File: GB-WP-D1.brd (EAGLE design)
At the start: 39.7 x 44.1 mm, 9 parts

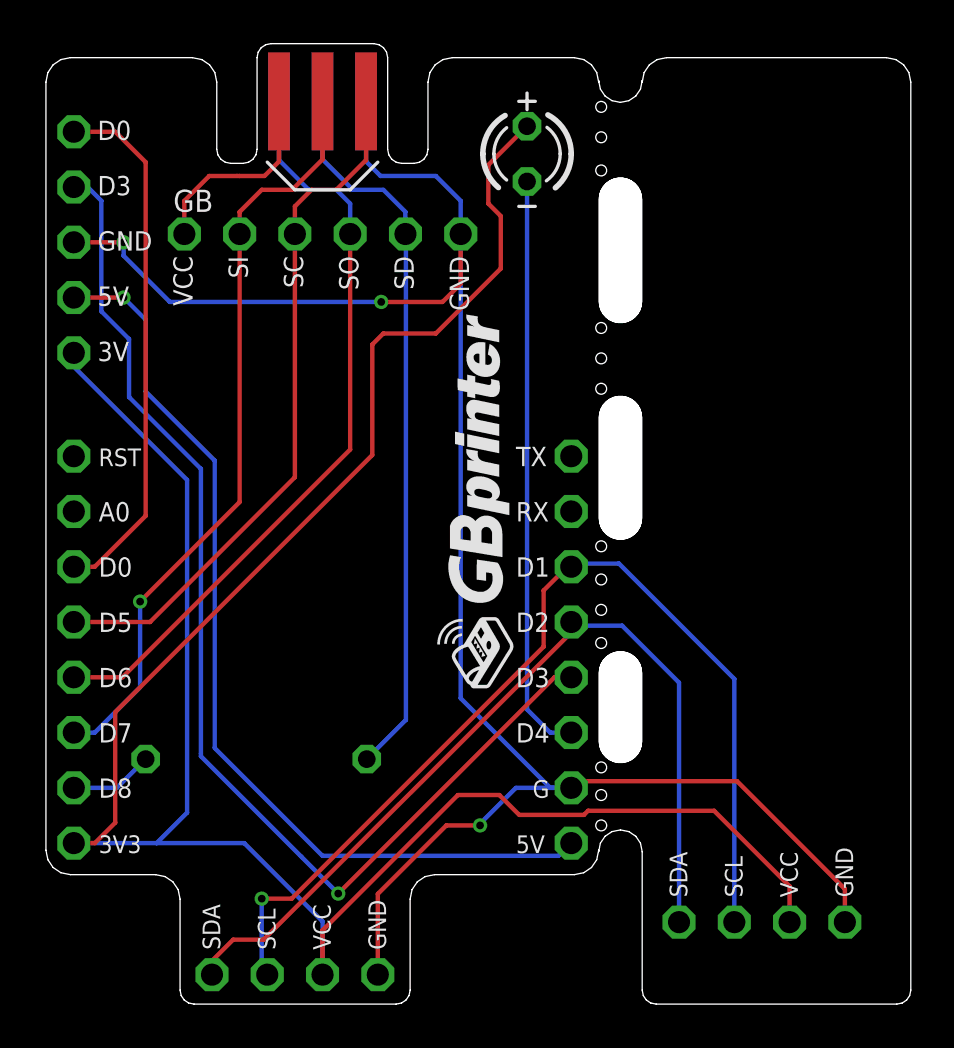
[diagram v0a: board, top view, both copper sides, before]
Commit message: Add files via upload
WEMOS D1 mini size
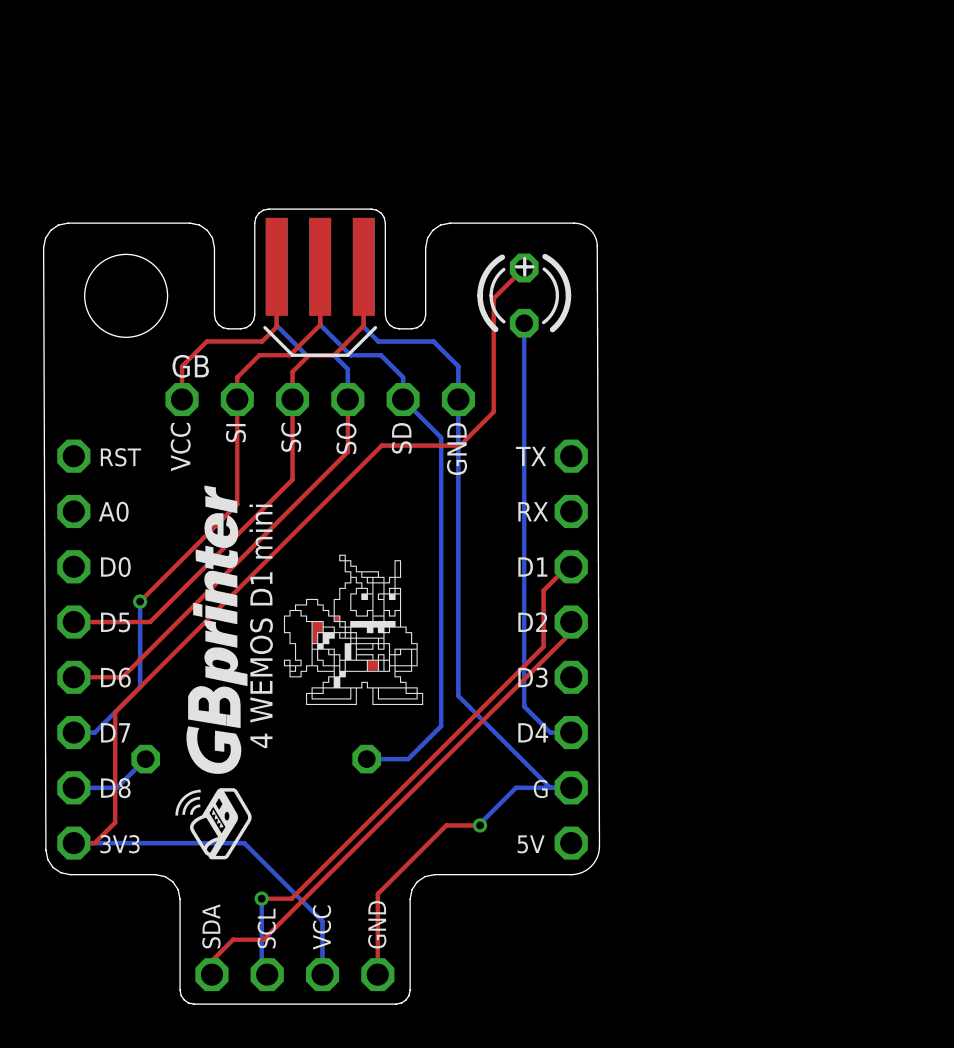
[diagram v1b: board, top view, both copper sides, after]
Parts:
- removed JP2: (no value), pinhead_v2:1X05/OCT
- removed JP5: (no value), pinhead_v2:1X04/OCT
- added U$3: KAMENRIDER_LOGOV2_COLOR_OPAC, kamenrider:10_6_V2
- moved JP4 7.61 mm to (12.6, 27.7)
- moved U$2 7.61 mm to (12.6, 33.8)
- moved LED1 6.52 mm to (22.0, 32.5)
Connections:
- net 3.3V: no longer JP2.5, JP5.3
- net 5V: no longer JP2.4
- net D0: no longer JP2.1
- net D2: no longer JP5.1
- net D3: no longer JP2.2
- net GND: no longer JP2.3, JP5.4
- net N$7: no longer JP5.2
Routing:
- net 3.3V: track 114.3 -> 53.0 mm
- net D3: track 52.7 -> 0.00 mm, vias 1 -> 0
- net GND: track 90.4 -> 44.6 mm, vias 3 -> 1
- net 5V: track 43.4 -> 0.00 mm, vias 1 -> 0
- net D0: track 24.4 -> 0.00 mm
- net N$7: track 46.6 -> 25.7 mm
- net D2: track 41.0 -> 23.9 mm
- net D7: track 35.1 -> 27.5 mm
- net D6: track 35.1 -> 27.5 mm
- net D5: track 32.2 -> 24.6 mm
- net D4: track 26.7 -> 20.3 mm
- net N$5: track 33.4 -> 28.3 mm
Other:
- board size 39.7 x 44.1 mm -> 25.5 x 36.5 mm
- board text added: "4 WEMOS D1 mini"
- board text added: "https://git.io/JJk92 https://bit.ly/gbccd https://git.io/JJWkr"
- board text removed: "3V"
- board text removed: "https://bit.ly/gbccd"
- board text removed: "https://git.io/JJk92"

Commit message: Add files via upload
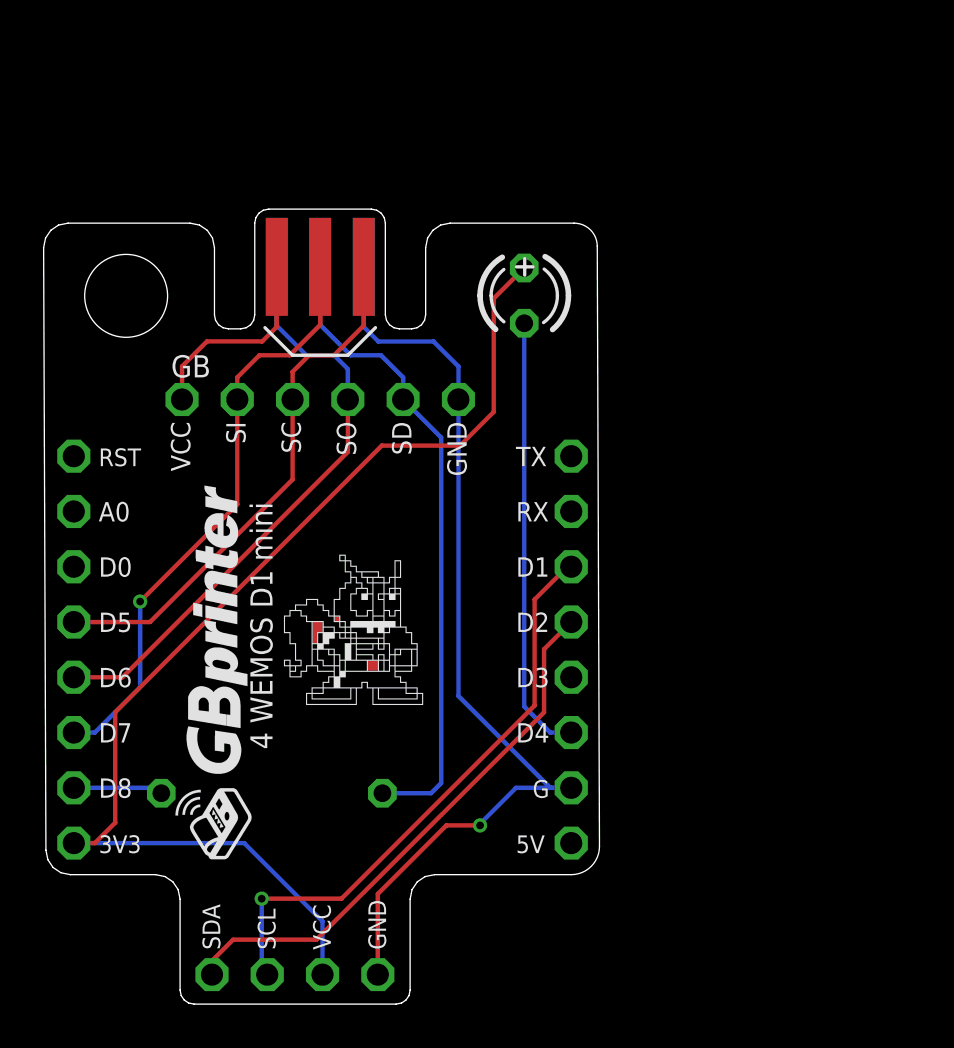
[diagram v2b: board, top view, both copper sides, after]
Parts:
- moved 4.7K 1.73 mm to (10.4, 9.61)
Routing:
- net N$5: track 28.3 -> 29.7 mm
- net D2: track 23.9 -> 25.3 mm
- net N$7: track 25.7 -> 27.0 mm
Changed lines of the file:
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@@
 <text x="13.081" y="2.413" size="0.8128" layer="21" font="vector" ratio="15" rot="R90">VCC</text>
 <text x="15.621" y="2.413" size="0.8128" layer="21" font="vector" ratio="15" rot="R90">GND</text>
-<text x="7.637584375" y="18.338246875" size="1.016" layer="22" ratio="12" rot="SMR270" align="center">https://git.io/JJk92
+<text x="7.192728125" y="17.109596875" size="0.762" layer="22" font="vector" ratio="12" distance="25" rot="SMR270" align="center">https://git.io/JJk92
 https://bit.ly/gbccd
 https://git.io/JJWkr</text>
@@
 </groups>
 <elements>
-<element name="4.7K" library="resistor" library_urn="urn:adsk.eagle:library:348" package="0207/10" package3d_urn="urn:adsk.eagle:package:23491/2" value="" x="9.652" y="11.176" smashed="yes" rot="SMR0">
-<attribute name="NAME" x="12.106859375" y="10.7617" size="1.016" layer="26" font="vector" ratio="15" rot="SMR0"/>
-<attribute name="VALUE" x="11.9126" y="10.541" size="1.27" layer="28" ratio="10" rot="SMR0"/>
+<element name="4.7K" library="resistor" library_urn="urn:adsk.eagle:library:348" package="0207/10" package3d_urn="urn:adsk.eagle:package:23491/2" value="" x="10.372240625" y="9.6084125" smashed="yes" rot="SMR0">
+<attribute name="NAME" x="12.8271" y="9.1941125" size="1.016" layer="26" font="vector" ratio="15" rot="SMR0"/>
+<attribute name="VALUE" x="12.632840625" y="8.9734125" size="1.27" layer="28" ratio="10" rot="SMR0"/>
 </element>
 <element name="U$2" library="link-port-pcb" package="GB-LINK-PCB" value="GB-LINK-PADS" x="12.594084375" y="33.7970875" smashed="yes"/>
@@
 <signal name="D2">
 <contactref element="JP1" pad="1"/>
-<wire x1="9.987215625" y1="2.878025" x2="8.593225" y2="2.878025" width="0.2032" layer="1"/>
+<wire x1="12.418403125" y1="2.878025" x2="8.593225" y2="2.878025" width="0.2032" layer="1"/>
 <wire x1="8.593225" y1="2.878025" x2="7.62" y2="1.9048" width="0.2032" layer="1"/>
 <wire x1="7.62" y1="1.27" x2="7.62" y2="1.9048" width="0.2032" layer="1"/>
-<wire x1="24.13" y1="16.997434375" x2="9.987215625" y2="2.878025" width="0.2032" layer="1"/>
+<wire x1="22.88016875" y1="13.322496875" x2="12.418403125" y2="2.878025" width="0.2032" layer="1"/>
 <contactref element="JP6" pad="4"/>
-<wire x1="24.13" y1="17.4752" x2="24.13" y2="16.997434375" width="0.2032" layer="1"/>
+<wire x1="24.13" y1="17.4752" x2="22.88016875" y2="16.22536875" width="0.2032" layer="1"/>
+<wire x1="22.88016875" y1="16.22536875" x2="22.88016875" y2="13.322496875" width="0.2032" layer="1"/>
 </signal>
 <signal name="D5">
@@
 <contactref element="4.7K" pad="2"/>
 <contactref element="JP3" pad="7"/>
-<wire x1="1.27" y1="9.8552" x2="3.2512" y2="9.8552" width="0.2032" layer="16"/>
-<wire x1="3.2512" y1="9.8552" x2="4.572" y2="11.176" width="0.2032" layer="16"/>
+<wire x1="1.27" y1="9.8552" x2="5.045453125" y2="9.8552" width="0.2032" layer="16"/>
+<wire x1="5.045453125" y1="9.8552" x2="5.292240625" y2="9.6084125" width="0.2032" layer="16"/>
 </signal>
 <signal name="D0">
@@
 <contactref element="4.7K" pad="1"/>
 <wire x1="16.404084375" y1="27.7010875" x2="18.152878125" y2="25.95229375" width="0.2032" layer="16"/>
-<wire x1="18.152878125" y1="12.690353125" x2="16.638525" y2="11.176" width="0.2032" layer="16"/>
-<wire x1="16.638525" y1="11.176" x2="14.732" y2="11.176" width="0.2032" layer="16"/>
-<wire x1="18.152878125" y1="25.95229375" x2="18.152878125" y2="12.690353125" width="0.2032" layer="16"/>
+<wire x1="18.152878125" y1="10.074178125" x2="17.6871125" y2="9.6084125" width="0.2032" layer="16"/>
+<wire x1="15.452240625" y1="9.6084125" x2="17.6871125" y2="9.6084125" width="0.2032" layer="16"/>
+<wire x1="18.152878125" y1="25.95229375" x2="18.152878125" y2="10.074178125" width="0.2032" layer="16"/>
 </signal>
 <signal name="N$7">
@@
 <wire x1="9.9061" y1="1.5239" x2="10.16" y2="1.27" width="0.2032" layer="16"/>
 <contactref element="JP6" pad="3"/>
-<wire x1="9.9061" y1="4.76236875" x2="11.2816875" y2="4.76236875" width="0.2032" layer="1"/>
-<wire x1="22.86" y1="16.34068125" x2="22.86" y2="18.923" width="0.2032" layer="1"/>
-<wire x1="22.86" y1="18.923" x2="23.9522" y2="20.0152" width="0.2032" layer="1"/>
+<wire x1="9.9061" y1="4.76236875" x2="13.569515625" y2="4.76236875" width="0.2032" layer="1"/>
+<wire x1="22.44691875" y1="13.639771875" x2="22.44691875" y2="18.50991875" width="0.2032" layer="1"/>
+<wire x1="22.44691875" y1="18.50991875" x2="23.9522" y2="20.0152" width="0.2032" layer="1"/>
 <wire x1="23.9522" y1="20.0152" x2="24.13" y2="20.0152" width="0.2032" layer="1"/>
-<wire x1="11.2816875" y1="4.76236875" x2="22.86" y2="16.34068125" width="0.2032" layer="1"/>
+<wire x1="13.569515625" y1="4.76236875" x2="22.44691875" y2="13.639771875" width="0.2032" layer="1"/>
 </signal>
 <signal name="A0">
